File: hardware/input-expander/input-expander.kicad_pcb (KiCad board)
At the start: 4 copper layers, 78.5 x 93 mm, 72 parts, among them J2 JTAG, J3 CONSOLE, J4 Delphi_Sicma_24, Q2 MBT3904DW1T1G, Q3 MBT3904DW1T1G, Q4 MBT3904DW1T1G, U2 SN65HVD230, U3 TLS850B0TEV33ATMA1, U4 TLS850F2TAV50ATMA1, U5 STM32G491CEU6

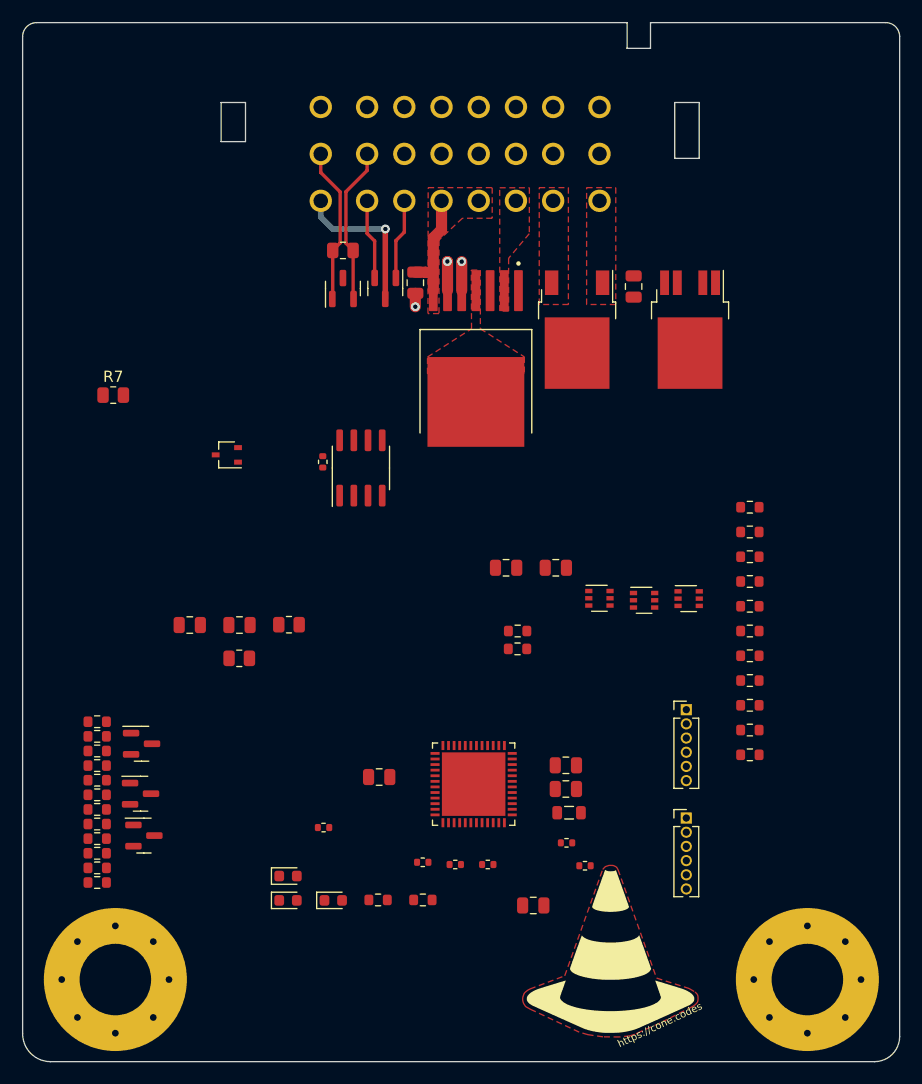
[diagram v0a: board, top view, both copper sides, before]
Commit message: u like resistors
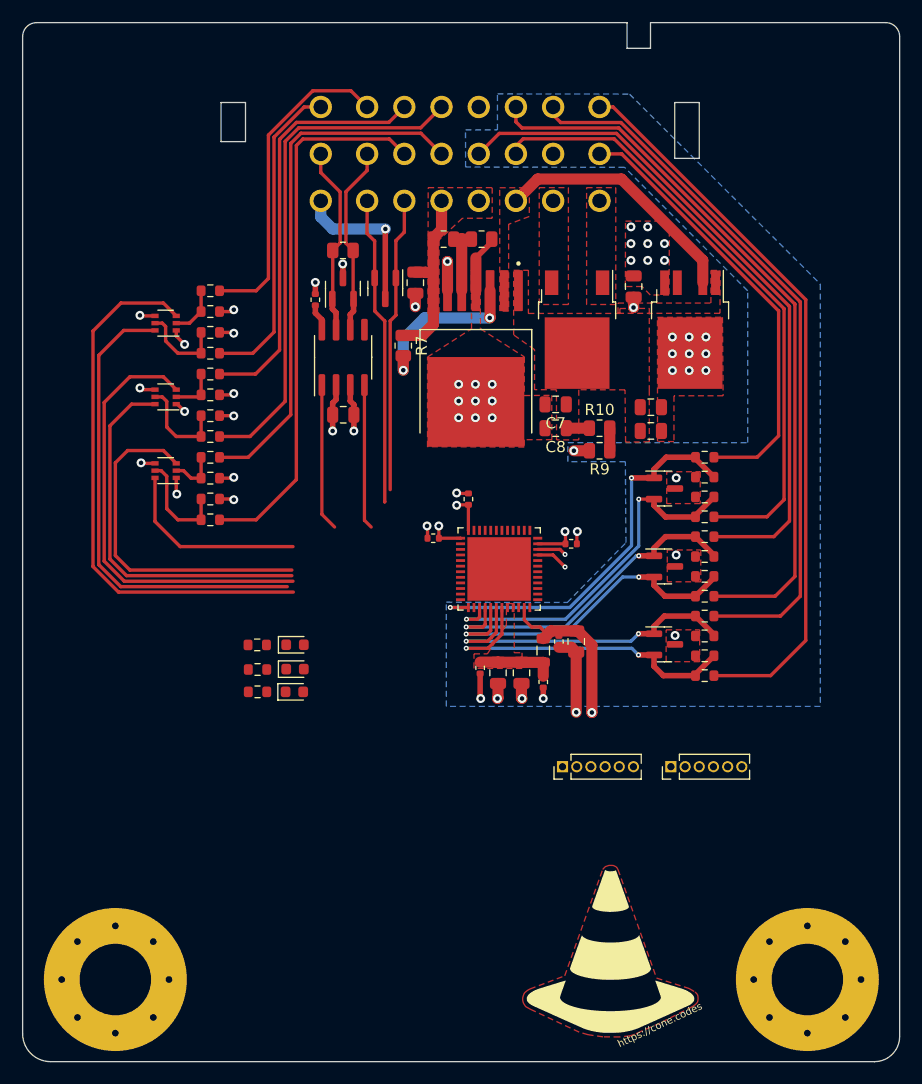
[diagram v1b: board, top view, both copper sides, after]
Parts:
- removed D6: BAT54AW,115, Package_TO_SOT_SMD:SOT-323_SC-70
- added R10: R_Small, Resistor_SMD:R_0805_2012Metric, F.Cu at (83.6, 60.8)
- added R9: R_Small, Resistor_SMD:R_0805_2012Metric, F.Cu at (83.6, 62.8)
- moved R36 62.5 mm to (48.8, 50.4), turned to 0 degrees
- moved R21 62.4 mm to (93.0, 67.0)
- moved R20 61.4 mm to (93.0, 65.2)
- moved R22 61.1 mm to (93.0, 72.3)
- moved R14 61.0 mm to (93.0, 63.4)
- moved R17 60.9 mm to (93.0, 68.7)
- moved R23 60.9 mm to (93.0, 74.1)
- moved R15 59.6 mm to (93.0, 70.5)
- moved R24 57.8 mm to (93.0, 79.4)
- moved R18 56.8 mm to (93.0, 75.8)
- moved R16 55.4 mm to (93.0, 77.6)
- moved R25 55.0 mm to (93.0, 81.2)
- moved R30 54.9 mm to (48.8, 48.5)
- moved R19 54.5 mm to (93.0, 83.0)
- moved R34 54.0 mm to (48.8, 61.5)
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- renumbered R9 to R11, R10 to R12, R11 to R13, R12 to R14, R13 to R15, R14 to R16, R15 to R17, R16 to R18, R17 to R19, R18 to R20, R19 to R21, R20 to R22, R21 to R23, R22 to R24, R23 to R25, R24 to R26, R25 to R27, R26 to R28, R27 to R29, R28 to R30, R29 to R31, R30 to R32, R31 to R33, R32 to R34, R33 to R35, R34 to R36, R35 to R37, R36 to R38, R37 to R39, R38 to R40, R39 to R41
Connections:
- D10 pad 1: /ADC_IN3 -> /ADC2_IN5
- D10 pad 2: /ADC_IN4 -> /ADC1_IN15
- D11 pad 1: /ADC_IN5 -> /ADC1_IN12
- D11 pad 2: /ADC_IN6 -> /ADC2_IN12
- D9 pad 1: /ADC_IN1 -> /ADC2_IN13
- D9 pad 2: /ADC_IN2 -> /ADC2_IN4
- J4 pad B3: /DIN1 -> /DIN6
- J4 pad B4: /DIN2 -> /DIN5
- J4 pad B5: /DIN3 -> /AIN3
- J4 pad B6: /DIN4 -> /AIN2
- J4 pad B7: /DIN5 -> GNDS
- J4 pad B8: /DIN6 -> /AIN1
- J4 pad C1: GNDPWR -> /DIN2
- J4 pad C2: GNDS -> /DIN1
- J4 pad C3: /AIN6 -> /DIN3
- J4 pad C4: /AIN5 -> /DIN4
- J4 pad C5: /AIN4 -> GNDPWR
- J4 pad C6: /AIN3 -> /AIN4
- J4 pad C7: /AIN2 -> /AIN5
- J4 pad C8: /AIN1 -> /AIN6
- R14 pad 1: /ADC_IN1 -> /ADC2_IN13
- R15 pad 1: /ADC_IN3 -> /ADC2_IN5
- R16 pad 1: /ADC_IN5 -> /ADC1_IN12
- R17 pad 1: /ADC_IN2 -> /ADC2_IN4
- R18 pad 1: /ADC_IN4 -> /ADC1_IN15
- R19 pad 1: /ADC_IN6 -> /ADC2_IN12
- R20 pad 2: /ADC_IN1 -> /ADC2_IN13
- R21 pad 2: /ADC_IN2 -> /ADC2_IN4
- R22 pad 2: /ADC_IN3 -> /ADC2_IN5
- R23 pad 2: /ADC_IN4 -> /ADC1_IN15
- R24 pad 2: /ADC_IN5 -> /ADC1_IN12
- R25 pad 2: /ADC_IN6 -> /ADC2_IN12
- R27 pad 1: GND -> GNDS
- R28 pad 1: GND -> GNDS
- U2 pad 1: /GPIO_CAN_P -> /FDCAN2_TX
- U2 pad 4: /GPIO_CAN_N -> /FDCAN2_RX
- U5 pad 11: unconnected-(U5-Pad11) -> /ADC1_IN4
- U5 pad 12: unconnected-(U5-Pad12) -> /ADC2_IN17
- U5 pad 13: unconnected-(U5-Pad13) -> /ADC2_IN13
- U5 pad 14: unconnected-(U5-Pad14) -> /ADC2_IN3
- U5 pad 15: unconnected-(U5-Pad15) -> /ADC2_IN4
- U5 pad 16: unconnected-(U5-Pad16) -> /ADC2_IN5
- U5 pad 17: unconnected-(U5-Pad17) -> /ADC1_IN15
- U5 pad 18: unconnected-(U5-Pad18) -> /ADC1_IN12
- U5 pad 19: unconnected-(U5-Pad19) -> /ADC2_IN12
- U5 pad 33: unconnected-(U5-Pad33) -> /USB_D-
- U5 pad 34: unconnected-(U5-Pad34) -> /USB_D+
- U5 pad 36: unconnected-(U5-Pad36) -> /SWDIO-JTMS
- U5 pad 37: unconnected-(U5-Pad37) -> /SWCLK-JTCK
- U5 pad 38: unconnected-(U5-Pad38) -> /JTDI
- U5 pad 40: unconnected-(U5-Pad40) -> /JTDO
- U5 pad 42: unconnected-(U5-Pad42) -> /FDCAN2_TX
- U5 pad 43: unconnected-(U5-Pad43) -> /FDCAN2_RX
- U5 pad 5: unconnected-(U5-Pad5) -> /ADC1_IN10
- U5 pad 6: unconnected-(U5-Pad6) -> /ADC2_IN10
- U5 pad 8: unconnected-(U5-Pad8) -> /ADC12_IN1
- U5 pad 9: unconnected-(U5-Pad9) -> /ADC12_IN2
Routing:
- net /AIN6: track 0.00 -> 65.6 mm
- net /AIN4: track 0.00 -> 65.4 mm
- net /AIN5: track 0.00 -> 64.6 mm
- net /AIN3: track 0.00 -> 61.5 mm
- net /AIN2: track 0.00 -> 55.3 mm
- net unconnected-(Q2-Pad3): track 0.00 -> 48.9 mm
- net /DIN6: track 0.00 -> 48.7 mm
- net /DIN5: track 0.00 -> 46.9 mm
- net /DIN4: track 0.00 -> 45.7 mm
- net unconnected-(Q2-Pad6): track 0.00 -> 42.4 mm
- net unconnected-(Q3-Pad3): track 0.00 -> 39.7 mm
- net /AIN1: track 0.00 -> 39.6 mm
- net GND: track 1.20 -> 40.3 mm, vias 1 -> 39
- net /DIN3: track 0.00 -> 37.5 mm
- net /ADC2_IN13: track 0.00 -> 35.6 mm, vias 0 -> 2
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- added copper zone on F.Cu, net +3V3
- added copper zone on F.Cu, net /VDDA
- added copper zone on F.Cu, net /VIN
- added copper zone on B.Cu, net GNDS
- added copper zone on F.Cu, net GNDS
- added copper zone on In1.Cu, net GNDS
- added copper zone on In2.Cu, net GNDS
